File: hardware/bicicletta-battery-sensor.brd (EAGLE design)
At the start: 45.7 x 19.1 mm, 24 parts, among them IC1 LMP92064, Q1 BSS138, Q2 BSS138, Q3 BSS138, Q4 BSS138

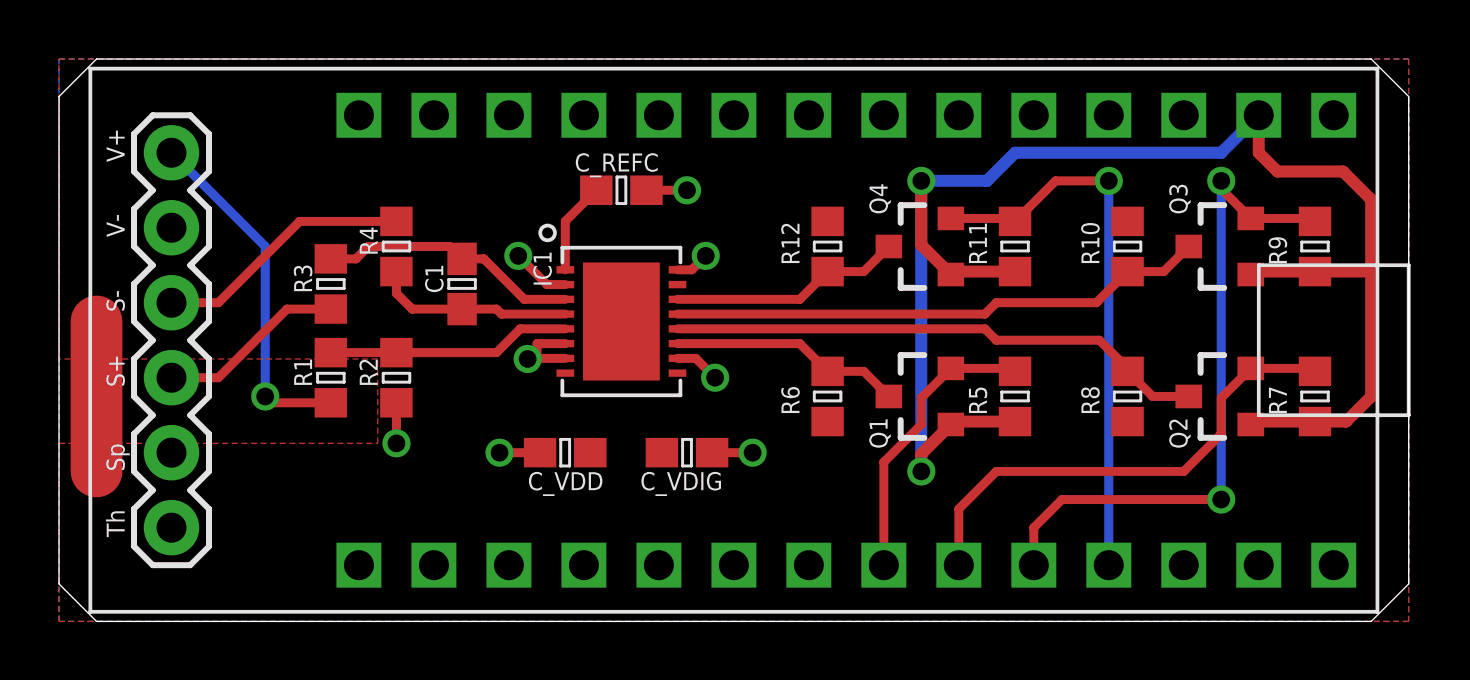
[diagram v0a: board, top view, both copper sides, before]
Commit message: Tidying some traces up.
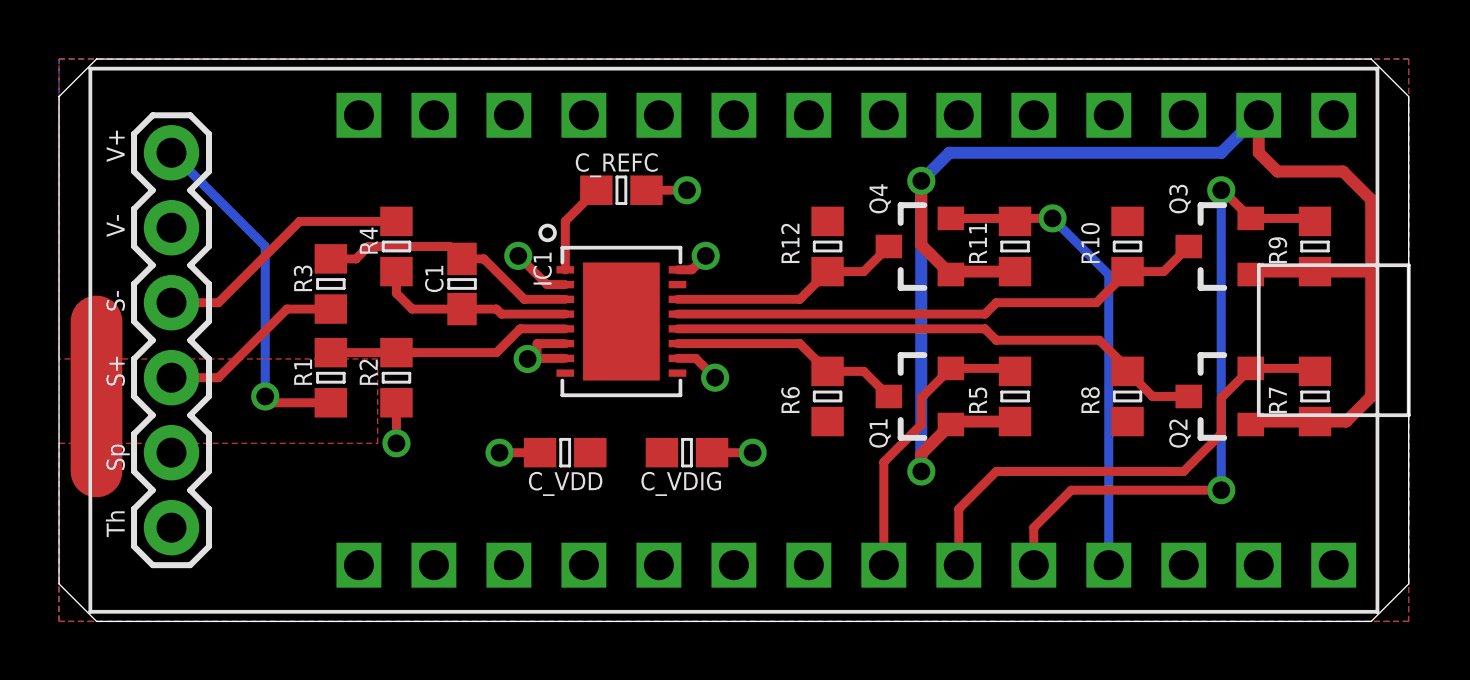
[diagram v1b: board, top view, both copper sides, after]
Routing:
- net SS: track 19.0 -> 16.1 mm
- net CLK: track 22.7 -> 21.9 mm
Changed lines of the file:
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@@
 <wire x1="42.445" y1="13.65" x2="42.545" y2="13.55" width="0.3048" layer="1"/>
 <wire x1="33.02" y1="1.905" x2="33.02" y2="3.175" width="0.3048" layer="1"/>
-<wire x1="33.02" y1="3.175" x2="33.9725" y2="4.1275" width="0.3048" layer="1"/>
-<wire x1="33.9725" y1="4.1275" x2="39.37" y2="4.1275" width="0.3048" layer="1"/>
-<via x="39.37" y="4.1275" extent="1-16" drill="0.6"/>
-<wire x1="39.37" y1="4.1275" x2="39.37" y2="14.9225" width="0.3048" layer="16"/>
-<via x="39.37" y="14.9225" extent="1-16" drill="0.6"/>
-<wire x1="40.37" y1="13.65" x2="39.37" y2="14.65" width="0.3048" layer="1"/>
-<wire x1="39.37" y1="14.65" x2="39.37" y2="14.9225" width="0.3048" layer="1"/>
+<wire x1="33.02" y1="3.175" x2="34.29" y2="4.445" width="0.3048" layer="1"/>
+<wire x1="34.29" y1="4.445" x2="39.37" y2="4.445" width="0.3048" layer="1"/>
+<via x="39.37" y="4.445" extent="1-16" drill="0.6"/>
+<via x="39.37" y="14.605" extent="1-16" drill="0.6"/>
+<wire x1="40.37" y1="13.65" x2="39.415" y2="14.605" width="0.3048" layer="1"/>
+<wire x1="39.415" y1="14.605" x2="39.37" y2="14.605" width="0.3048" layer="1"/>
+<wire x1="39.37" y1="14.605" x2="39.37" y2="4.445" width="0.3048" layer="16"/>
 </signal>
 <signal name="SS">
@@
 <contactref element="Q4" pad="2"/>
 <contactref element="R11" pad="1"/>
-<wire x1="35.56" y1="1.905" x2="35.56" y2="14.9225" width="0.3048" layer="16"/>
-<via x="35.56" y="14.9225" extent="1-16" drill="0.6"/>
-<wire x1="35.56" y1="14.9225" x2="33.7575" y2="14.9225" width="0.3048" layer="1"/>
-<wire x1="33.7575" y1="14.9225" x2="32.385" y2="13.55" width="0.3048" layer="1"/>
+<via x="33.655" y="13.6525" extent="1-16" drill="0.6"/>
 <wire x1="30.21" y1="13.65" x2="32.285" y2="13.65" width="0.3048" layer="1"/>
 <wire x1="32.285" y1="13.65" x2="32.385" y2="13.55" width="0.3048" layer="1"/>
+<wire x1="32.385" y1="13.55" x2="32.4875" y2="13.6525" width="0.3048" layer="1"/>
+<wire x1="32.4875" y1="13.6525" x2="33.655" y2="13.6525" width="0.3048" layer="1"/>
+<wire x1="33.655" y1="13.6525" x2="35.56" y2="11.7475" width="0.3048" layer="16"/>
+<wire x1="35.56" y1="11.7475" x2="35.56" y2="1.905" width="0.3048" layer="16"/>
 </signal>
 <signal name="~D9/A9">
@@
 <wire x1="29.21" y1="5.08" x2="29.21" y2="14.9225" width="0.4064" layer="16"/>
 <via x="29.21" y="14.9225" extent="1-16" drill="0.6"/>
-<wire x1="31.4325" y1="14.9225" x2="32.385" y2="15.875" width="0.4064" layer="16"/>
-<wire x1="32.385" y1="15.875" x2="39.37" y2="15.875" width="0.4064" layer="16"/>
+<wire x1="29.21" y1="14.9225" x2="30.1625" y2="15.875" width="0.4064" layer="16"/>
+<wire x1="30.1625" y1="15.875" x2="39.37" y2="15.875" width="0.4064" layer="16"/>
 <wire x1="39.37" y1="15.875" x2="40.64" y2="17.145" width="0.4064" layer="16"/>
-<wire x1="31.4325" y1="14.9225" x2="29.21" y2="14.9225" width="0.4064" layer="16"/>
 <wire x1="30.21" y1="6.67" x2="29.21" y2="5.67" width="0.4064" layer="1"/>
 <wire x1="29.21" y1="5.67" x2="29.21" y2="5.08" width="0.4064" layer="1"/>
@@
 </signal>
 </signals>
+<errors>
+</errors>
 </board>
 </drawing>
